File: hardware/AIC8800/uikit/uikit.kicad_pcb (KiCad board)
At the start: 2 copper layers, 50.8 x 69.2 mm, 40 parts, among them J1 Conn_01x20, J2 Conn_01x20, J3 Conn_01x10, J4 Conn_01x06, J5 USB_C_Receptacle_USB2.0, J6 Micro_SD_Card_Det, J7 PJ-393-USA, U1 AIC1000A, U2 CH340N

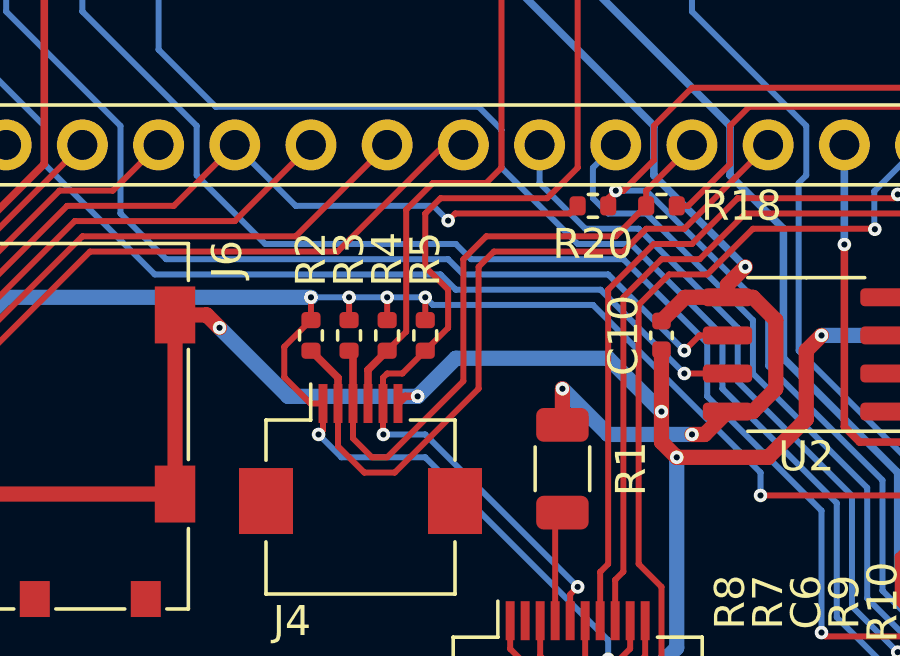
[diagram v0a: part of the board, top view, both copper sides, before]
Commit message: [hardware/AIC8800/uikit] minor tweak
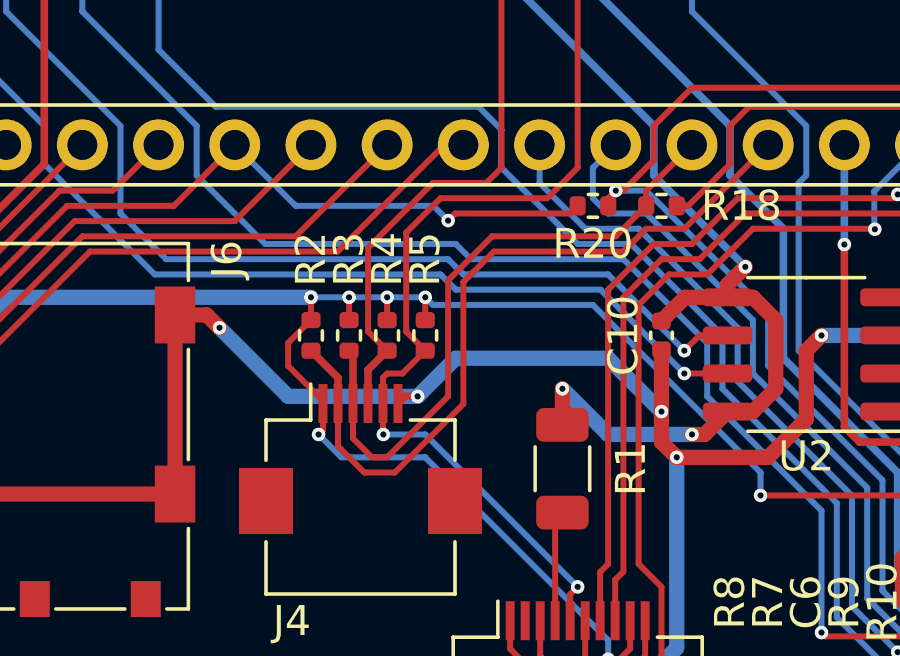
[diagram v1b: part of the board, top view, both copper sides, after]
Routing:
- net /B2: track 40.6 -> 41.1 mm
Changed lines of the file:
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@@
   (segment (start 243.84 129.54) (end 243.84 130.3) (width 0.254) (layer "F.Cu") (net 8))
   (segment (start 230.35 131.43) (end 230.35 132.362) (width 0.2) (layer "F.Cu") (net 8))
-  (segment (start 218.821 123.317) (end 218.821 122.299) (width 0.2) (layer "F.Cu") (net 8))
+  (segment (start 218.948 122.172) (end 219.71 121.41) (width 0.2) (layer "F.Cu") (net 8))
   (segment (start 220.111 124.191) (end 220.111 125.075) (width 0.2) (layer "F.Cu") (net 8))
   (segment (start 205.427 124.773) (end 205.74 124.46) (width 0.508) (layer "F.Cu") (net 8))
-  (segment (start 218.821 122.299) (end 219.71 121.41) (width 0.2) (layer "F.Cu") (net 8))
   (segment (start 229.997 132.715) (end 229.616 132.715) (width 0.2) (layer "F.Cu") (net 8))
   (segment (start 223.52 121.41) (end 223.52 120.65) (width 0.2) (layer "F.Cu") (net 8))
   (segment (start 244.52 135.02) (end 246.135 135.02) (width 0.2) (layer "F.Cu") (net 8))
+  (segment (start 218.948 122.936) (end 218.948 122.172) (width 0.2) (layer "F.Cu") (net 8))
   (segment (start 241.3 128.778) (end 241.3 129.54) (width 0.2) (layer "F.Cu") (net 8))
   (segment (start 246.535 134.62) (end 246.535 134.194479) (width 0.2) (layer "F.Cu") (net 8))
@@
   (segment (start 230.35 132.362) (end 229.997 132.715) (width 0.2) (layer "F.Cu") (net 8))
   (segment (start 220.111 125.075) (end 219.964 125.222) (width 0.2) (layer "F.Cu") (net 8))
-  (segment (start 220.111 124.191) (end 219.695 124.191) (width 0.2) (layer "F.Cu") (net 8))
   (segment (start 241.3 130.3) (end 241.3 129.54) (width 0.2) (layer "F.Cu") (net 8))
+  (segment (start 220.111 124.191) (end 220.111 124.099) (width 0.2) (layer "F.Cu") (net 8))
   (segment (start 239.776 127.254) (end 241.3 128.778) (width 0.2) (layer "F.Cu") (net 8))
   (segment (start 210.82 116.205) (end 207.645 119.38) (width 0.254) (layer "F.Cu") (net 8))
   (segment (start 246.135 135.02) (end 246.535 134.62) (width 0.2) (layer "F.Cu") (net 8))
-  (segment (start 219.695 124.191) (end 218.821 123.317) (width 0.2) (layer "F.Cu") (net 8))
+  (segment (start 220.111 124.099) (end 218.948 122.936) (width 0.2) (layer "F.Cu") (net 8))
   (via (at 219.964 125.222) (size 0.45212) (drill 0.2032) (layers "F.Cu" "B.Cu") (net 8))
   (via (at 241.3 129.54) (size 0.45212) (drill 0.2032) (layers "F.Cu" "B.Cu") (net 8))
@@
   (segment (start 222.111 123.329) (end 222.25 123.19) (width 0.2) (layer "F.Cu") (net 22))
   (segment (start 228.35 131.43) (end 228.35 130.552) (width 0.2) (layer "F.Cu") (net 22))
-  (segment (start 224.028 117.348) (end 223.52 117.856) (width 0.2) (layer "F.Cu") (net 22))
-  (segment (start 224.282 121.668) (end 223.52 122.43) (width 0.2) (layer "F.Cu") (net 22))
+  (segment (start 223.52 122.43) (end 222.885 121.795) (width 0.2) (layer "F.Cu") (net 22))
   (segment (start 222.123 125.222) (end 222.111 125.21) (width 0.2) (layer "F.Cu") (net 22))
   (segment (start 228.6 116.332) (end 227.584 117.348) (width 0.2) (layer "F.Cu") (net 22))
   (segment (start 227.584 117.348) (end 224.028 117.348) (width 0.2) (layer "F.Cu") (net 22))
-  (segment (start 223.52 119.634) (end 224.282 120.396) (width 0.2) (layer "F.Cu") (net 22))
   (segment (start 228.35 130.552) (end 228.6 130.302) (width 0.2) (layer "F.Cu") (net 22))
   (segment (start 223.518 122.43) (end 223.52 122.43) (width 0.2) (layer "F.Cu") (net 22))
   (segment (start 222.111 124.191) (end 222.111 123.329) (width 0.2) (layer "F.Cu") (net 22))
+  (segment (start 222.885 118.491) (end 224.028 117.348) (width 0.2) (layer "F.Cu") (net 22))
   (segment (start 222.25 123.19) (end 222.758 123.19) (width 0.2) (layer "F.Cu") (net 22))
+  (segment (start 222.885 121.795) (end 222.885 118.491) (width 0.2) (layer "F.Cu") (net 22))
   (segment (start 222.758 123.19) (end 223.518 122.43) (width 0.2) (layer "F.Cu") (net 22))
-  (segment (start 223.52 117.856) (end 223.52 119.634) (width 0.2) (layer "F.Cu") (net 22))
   (segment (start 228.6 99.06) (end 228.6 116.332) (width 0.2) (layer "F.Cu") (net 22))
   (segment (start 222.111 125.21) (end 222.111 124.191) (width 0.2) (layer "F.Cu") (net 22))
-  (segment (start 224.282 120.396) (end 224.282 121.668) (width 0.2) (layer "F.Cu") (net 22))
   (segment (start 237.49 90.17) (end 228.6 99.06) (width 0.2) (layer "F.Cu") (net 22))
   (via (at 222.123 125.222) (size 0.45212) (drill 0.2032) (layers "F.Cu" "B.Cu") (net 22))
@@
   (segment (start 223.52 125.222) (end 222.123 125.222) (width 0.2) (layer "B.Cu") (net 22))
   (segment (start 228.6 130.302) (end 223.52 125.222) (width 0.2) (layer "B.Cu") (net 22))
-  (segment (start 223.774 116.84) (end 222.885 117.729) (width 0.2) (layer "F.Cu") (net 23))
-  (segment (start 222.885 117.729) (end 222.885 121.795) (width 0.2) (layer "F.Cu") (net 23))
+  (segment (start 222.25 122.43) (end 221.615 121.795) (width 0.2) (layer "F.Cu") (net 23))
   (segment (start 226.06 99.06) (end 226.06 116.332) (width 0.2) (layer "F.Cu") (net 23))
   (segment (start 221.611 124.191) (end 221.611 123.069) (width 0.254) (layer "F.Cu") (net 23))
+  (segment (start 221.615 118.999) (end 223.774 116.84) (width 0.2) (layer "F.Cu") (net 23))
+  (segment (start 221.615 121.795) (end 221.615 118.999) (width 0.2) (layer "F.Cu") (net 23))
   (segment (start 234.95 90.17) (end 226.06 99.06) (width 0.2) (layer "F.Cu") (net 23))
   (segment (start 226.06 116.332) (end 225.552 116.84) (width 0.2) (layer "F.Cu") (net 23))
   (segment (start 221.611 123.069) (end 222.25 122.43) (width 0.254) (layer "F.Cu") (net 23))
-  (segment (start 222.885 121.795) (end 222.25 122.43) (width 0.2) (layer "F.Cu") (net 23))
   (segment (start 225.552 116.84) (end 223.774 116.84) (width 0.2) (layer "F.Cu") (net 23))
   (segment (start 241.3 131.369975) (end 242.17 132.239975) (width 0.2) (layer "F.Cu") (net 24))
@@
   (segment (start 238.506 118.38156) (end 238.48794 118.3635) (width 0.2) (layer "B.Cu") (net 37))
   (segment (start 230.124 119.126) (end 225.806 119.126) (width 0.2) (layer "F.Cu") (net 38))
-  (segment (start 221.488 126.492) (end 220.611 125.615) (width 0.2) (layer "F.Cu") (net 38))
+  (segment (start 225.806 119.126) (end 224.79 120.142) (width 0.2) (layer "F.Cu") (net 38))
   (segment (start 220.611 124.191) (end 220.611 123.331) (width 0.254) (layer "F.Cu") (net 38))
   (segment (start 230.886 118.364) (end 230.124 119.126) (width 0.2) (layer "F.Cu") (net 38))
+  (segment (start 234.95 115.57) (end 232.156 118.364) (width 0.2) (layer "F.Cu") (net 38))
   (segment (start 220.611 123.331) (end 219.71 122.43) (width 0.254) (layer "F.Cu") (net 38))
-  (segment (start 225.806 119.126) (end 225.298 119.634) (width 0.2) (layer "F.Cu") (net 38))
-  (segment (start 225.298 119.634) (end 225.298 123.698) (width 0.2) (layer "F.Cu") (net 38))
-  (segment (start 225.298 123.698) (end 222.504 126.492) (width 0.2) (layer "F.Cu") (net 38))
-  (segment (start 234.95 115.57) (end 232.156 118.364) (width 0.2) (layer "F.Cu") (net 38))
+  (segment (start 224.79 120.142) (end 224.79 124.206) (width 0.2) (layer "F.Cu") (net 38))
+  (segment (start 222.504 126.492) (end 221.488 126.492) (width 0.2) (layer "F.Cu") (net 38))
+  (segment (start 224.79 124.206) (end 222.504 126.492) (width 0.2) (layer "F.Cu") (net 38))
   (segment (start 220.611 125.615) (end 220.611 124.191) (width 0.2) (layer "F.Cu") (net 38))
-  (segment (start 222.504 126.492) (end 221.488 126.492) (width 0.2) (layer "F.Cu") (net 38))
+  (segment (start 221.488 126.492) (end 220.611 125.615) (width 0.2) (layer "F.Cu") (net 38))
   (segment (start 232.156 118.364) (end 230.886 118.364) (width 0.2) (layer "F.Cu") (net 38))
-  (segment (start 229.868 118.618) (end 225.552 118.618) (width 0.2) (layer "F.Cu") (net 39))
-  (segment (start 224.79 123.444) (end 222.25 125.984) (width 0.2) (layer "F.Cu") (net 39))
-  (segment (start 224.79 119.38) (end 224.79 123.444) (width 0.2) (layer "F.Cu") (net 39))
   (segment (start 221.111 125.353) (end 221.111 124.191) (width 0.2) (layer "F.Cu") (net 39))
+  (segment (start 221.742 125.984) (end 221.111 125.353) (width 0.2) (layer "F.Cu") (net 39))
+  (segment (start 224.282 120.084315) (end 224.282 123.952) (width 0.2) (layer "F.Cu") (net 39))
+  (segment (start 221.111 122.561) (end 220.98 122.43) (width 0.254) (layer "F.Cu") (net 39))
+  (segment (start 230.884 117.602) (end 229.868 118.618) (width 0.2) (layer "F.Cu") (net 39))
+  (segment (start 224.282 123.952) (end 222.25 125.984) (width 0.2) (layer "F.Cu") (net 39))
+  (segment (start 221.111 124.191) (end 221.111 122.561) (width 0.254) (layer "F.Cu") (net 39))
+  (segment (start 225.748315 118.618) (end 224.282 120.084315) (width 0.2) (layer "F.Cu") (net 39))
+  (segment (start 230.884 117.096) (end 230.884 117.602) (width 0.2) (layer "F.Cu") (net 39))
+  (segment (start 229.868 118.618) (end 225.748315 118.618) (width 0.2) (layer "F.Cu") (net 39))
   (segment (start 222.25 125.984) (end 221.742 125.984) (width 0.2) (layer "F.Cu") (net 39))
-  (segment (start 221.111 122.561) (end 220.98 122.43) (width 0.254) (layer "F.Cu") (net 39))
-  (segment (start 225.552 118.618) (end 224.79 119.38) (width 0.2) (layer "F.Cu") (net 39))
-  (segment (start 230.884 117.602) (end 229.868 118.618) (width 0.2) (layer "F.Cu") (net 39))
-  (segment (start 221.111 124.191) (end 221.111 122.561) (width 0.254) (layer "F.Cu") (net 39))
-  (segment (start 230.884 117.096) (end 230.884 117.602) (width 0.2) (layer "F.Cu") (net 39))
-  (segment (start 221.742 125.984) (end 221.111 125.353) (width 0.2) (layer "F.Cu") (net 39))
   (segment (start 232.41 115.57) (end 230.884 117.096) (width 0.2) (layer "F.Cu") (net 39))
   (segment (start 244.094 132.969) (end 243.971 132.969) (width 0.2) (layer "F.Cu") (net 40))
